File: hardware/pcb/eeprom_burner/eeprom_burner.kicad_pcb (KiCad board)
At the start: 2 copper layers, 68.6 x 53.3 mm, 23 parts, among them J1 Conn_01x08, J2 Conn_01x08, J3 Conn_01x08, J4 Conn_01x06, P1 Power, P2 Analog, P3 Digital, P4 Digital, P5 CONN_01X01, P6 CONN_01X01, P7 CONN_01X01, P8 CONN_01X01, U1 74HC595, U2 74HC595, U3 28C256, U4 28C256J

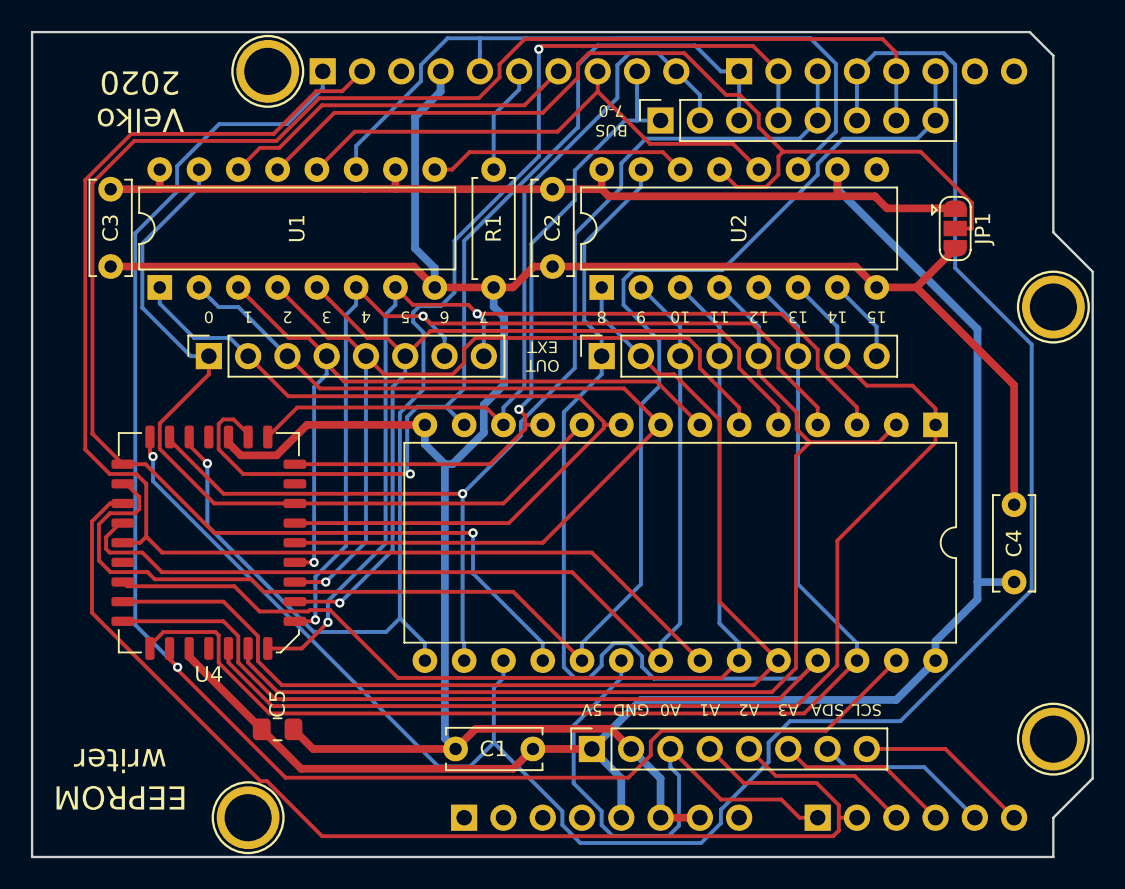
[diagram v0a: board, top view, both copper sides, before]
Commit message: Add copper pour
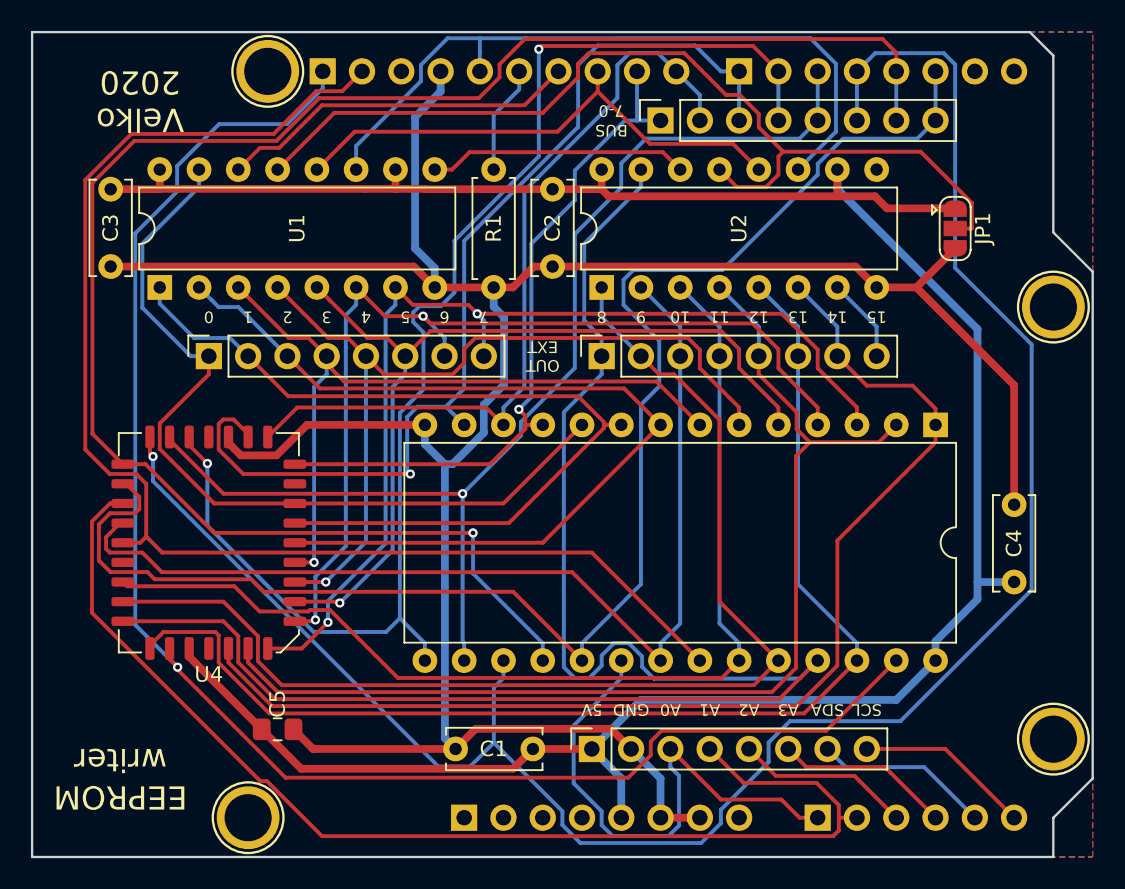
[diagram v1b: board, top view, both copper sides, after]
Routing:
- added copper zone on F.Cu, net +5V
- added copper zone on B.Cu, net GND
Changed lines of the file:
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@@
   (layers
     (0 F.Cu signal)
-    (31 B.Cu signal)
+    (31 B.Cu signal hide)
     (32 B.Adhes user hide)
     (33 F.Adhes user hide)
@@
     (42 Eco1.User user hide)
     (43 Eco2.User user hide)
-    (44 Edge.Cuts user hide)
+    (44 Edge.Cuts user)
     (45 Margin user hide)
     (46 B.CrtYd user hide)
@@
   (segment (start 118.3805 105.651) (end 119.4094 106.6799) (width 0.25) (layer F.Cu) (net 57))
   (segment (start 119.4094 106.6799) (end 147.1929 106.6799) (width 0.25) (layer F.Cu) (net 57))
+  (zone (net 2) (net_name GND) (layer B.Cu) (hatch edge 0.508)
+    (connect_pads (clearance 0.208))
+    (min_thickness 0.254)
+    (fill yes (arc_segments 16) (thermal_gap 0.508) (thermal_bridge_width 0.508))
+    (polygon
+      (pts
+        (xy 110.998 126.365) (xy 179.578 126.365) (xy 179.578 73.025) (xy 110.998 73.025)
+      )
+    )
+  )
+  (zone (net 1) (net_name +5V) (layer F.Cu) (hatch edge 0.508)
+    (connect_pads (clearance 0.208))
+    (min_thickness 0.254)
+    (fill yes (arc_segments 16) (thermal_gap 0.508) (thermal_bridge_width 0.508))
+    (polygon
+      (pts
+        (xy 110.998 126.365) (xy 179.578 126.365) (xy 179.578 73.025) (xy 110.998 73.025)
+      )
+    )
+  )
 )
